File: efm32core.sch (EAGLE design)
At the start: 5 parts

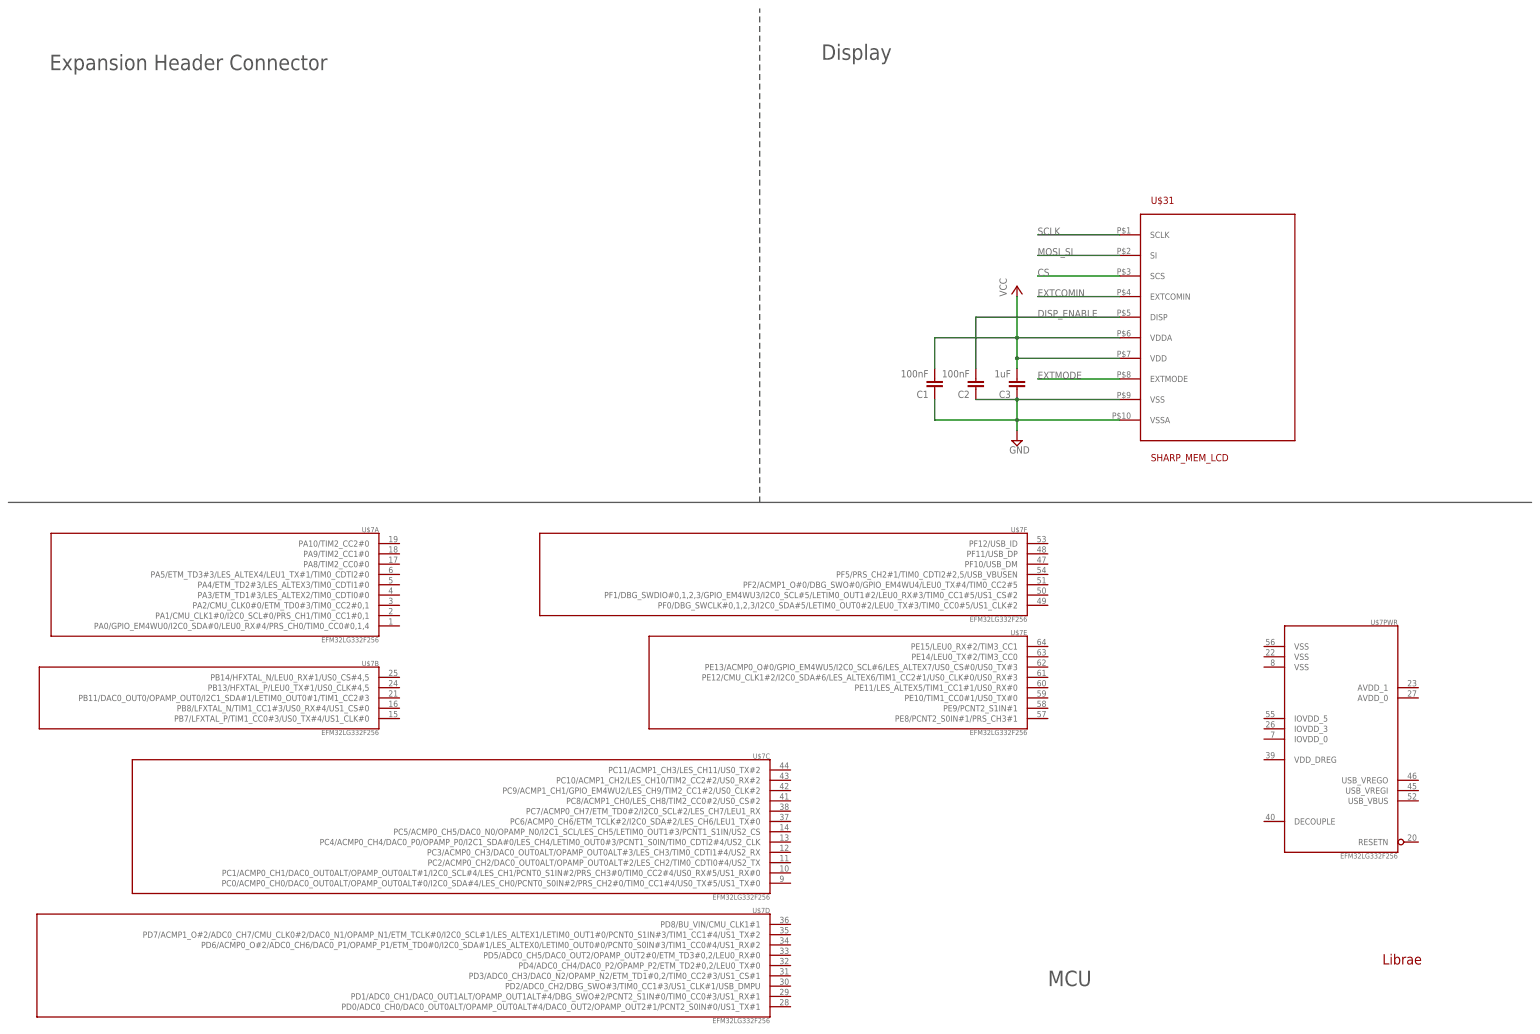
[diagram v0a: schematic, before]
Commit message: do cleanups, draw frame
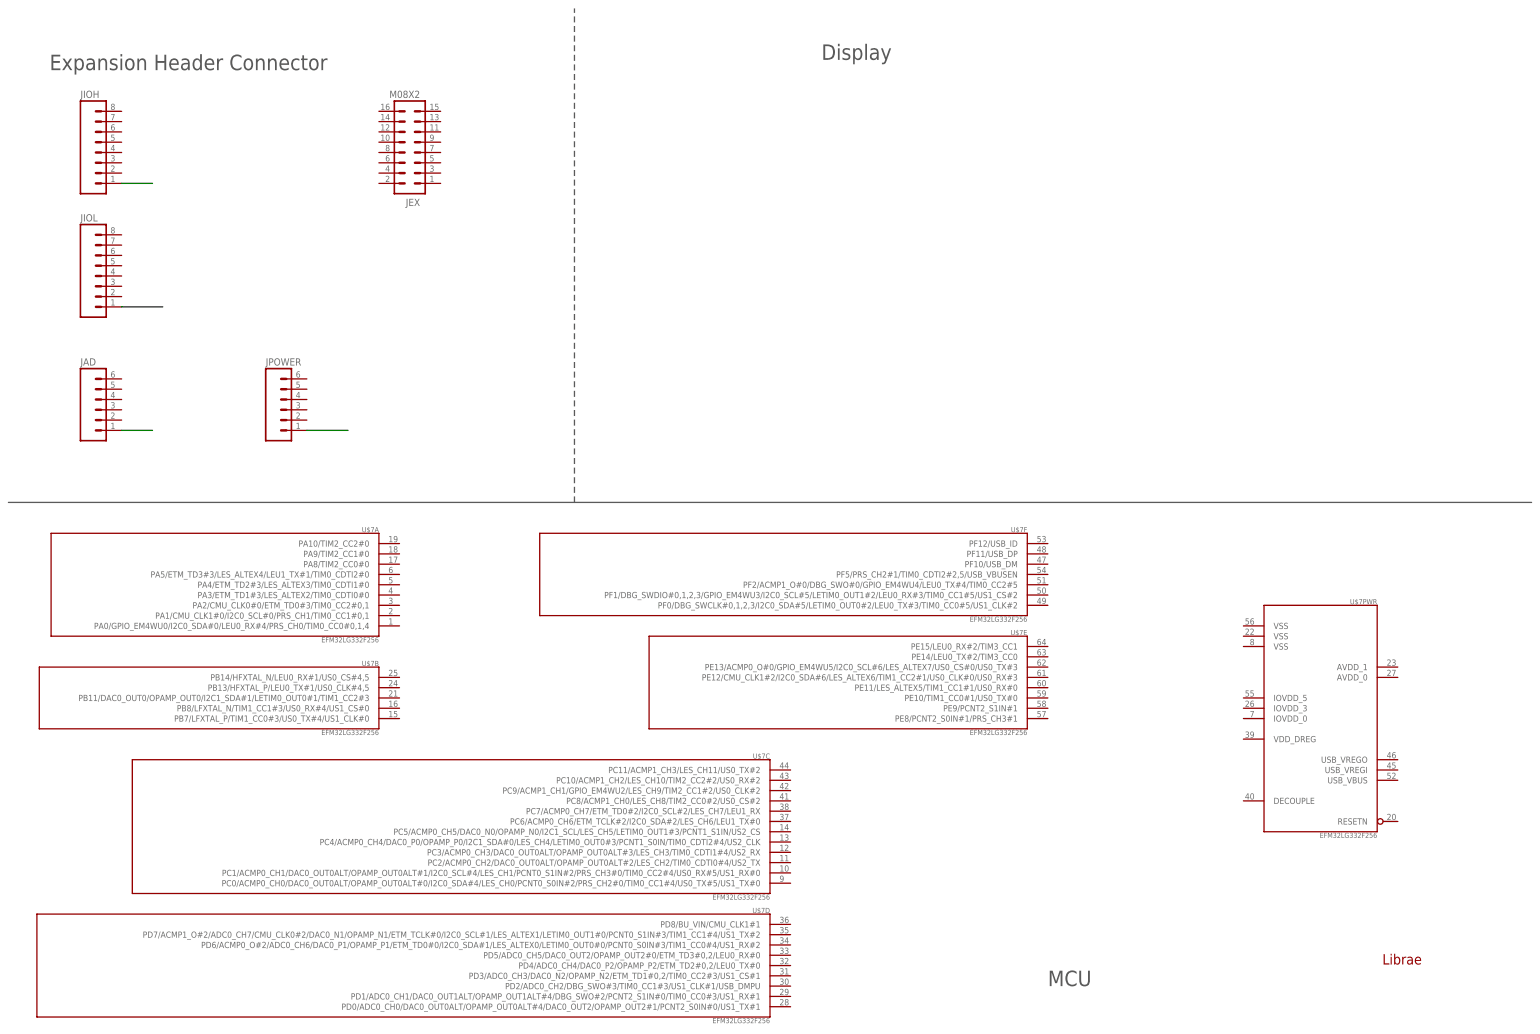
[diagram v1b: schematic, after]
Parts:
- removed C1, C2: 100nF, rcl:C-EUC0402K
- removed C3: 1uF, rcl:C-EUC0402K
- removed U$31: SHARP_MEM_LCD, sharp_mem_lcd:SHARP_MEM_LCD
- added JAD, JPOWER: (no value), SparkFun-Connectors:M06SIP
- added JEX: M08X2, SparkFun-Connectors:M08X2
- added JIOH, JIOL: (no value), SparkFun-Connectors:M081X08
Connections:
- removed net CS: U$31.SCS
- removed net DISP_ENABLE: C2.2, U$31.DISP
- removed net EXTCOMIN: U$31.EXTCOMIN
- removed net EXTMODE: U$31.EXTMODE
- removed net GND: C1.1, C2.1, C3.1, U$31.VSS, U$31.VSSA
- removed net MOSI_SI: U$31.SI
- removed net SCLK: U$31.SCLK
- removed net VCC: C1.2, C3.2, U$31.VDD, U$31.VDDA
- new net N$1: JIOH.1
- new net N$2: JAD.1
- new net N$3: JIOL.1
- new net N$4: JPOWER.1
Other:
- moved on the sheet: U$7PWR
